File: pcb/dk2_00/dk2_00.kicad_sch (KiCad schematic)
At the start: 6 parts, among them J1 Micro_SD_Card, J7 Conn_01x01_Pin, J8 Conn_01x01_Pin, J9 Conn_01x01_Pin, SW1 SW_Push, U1 Pico

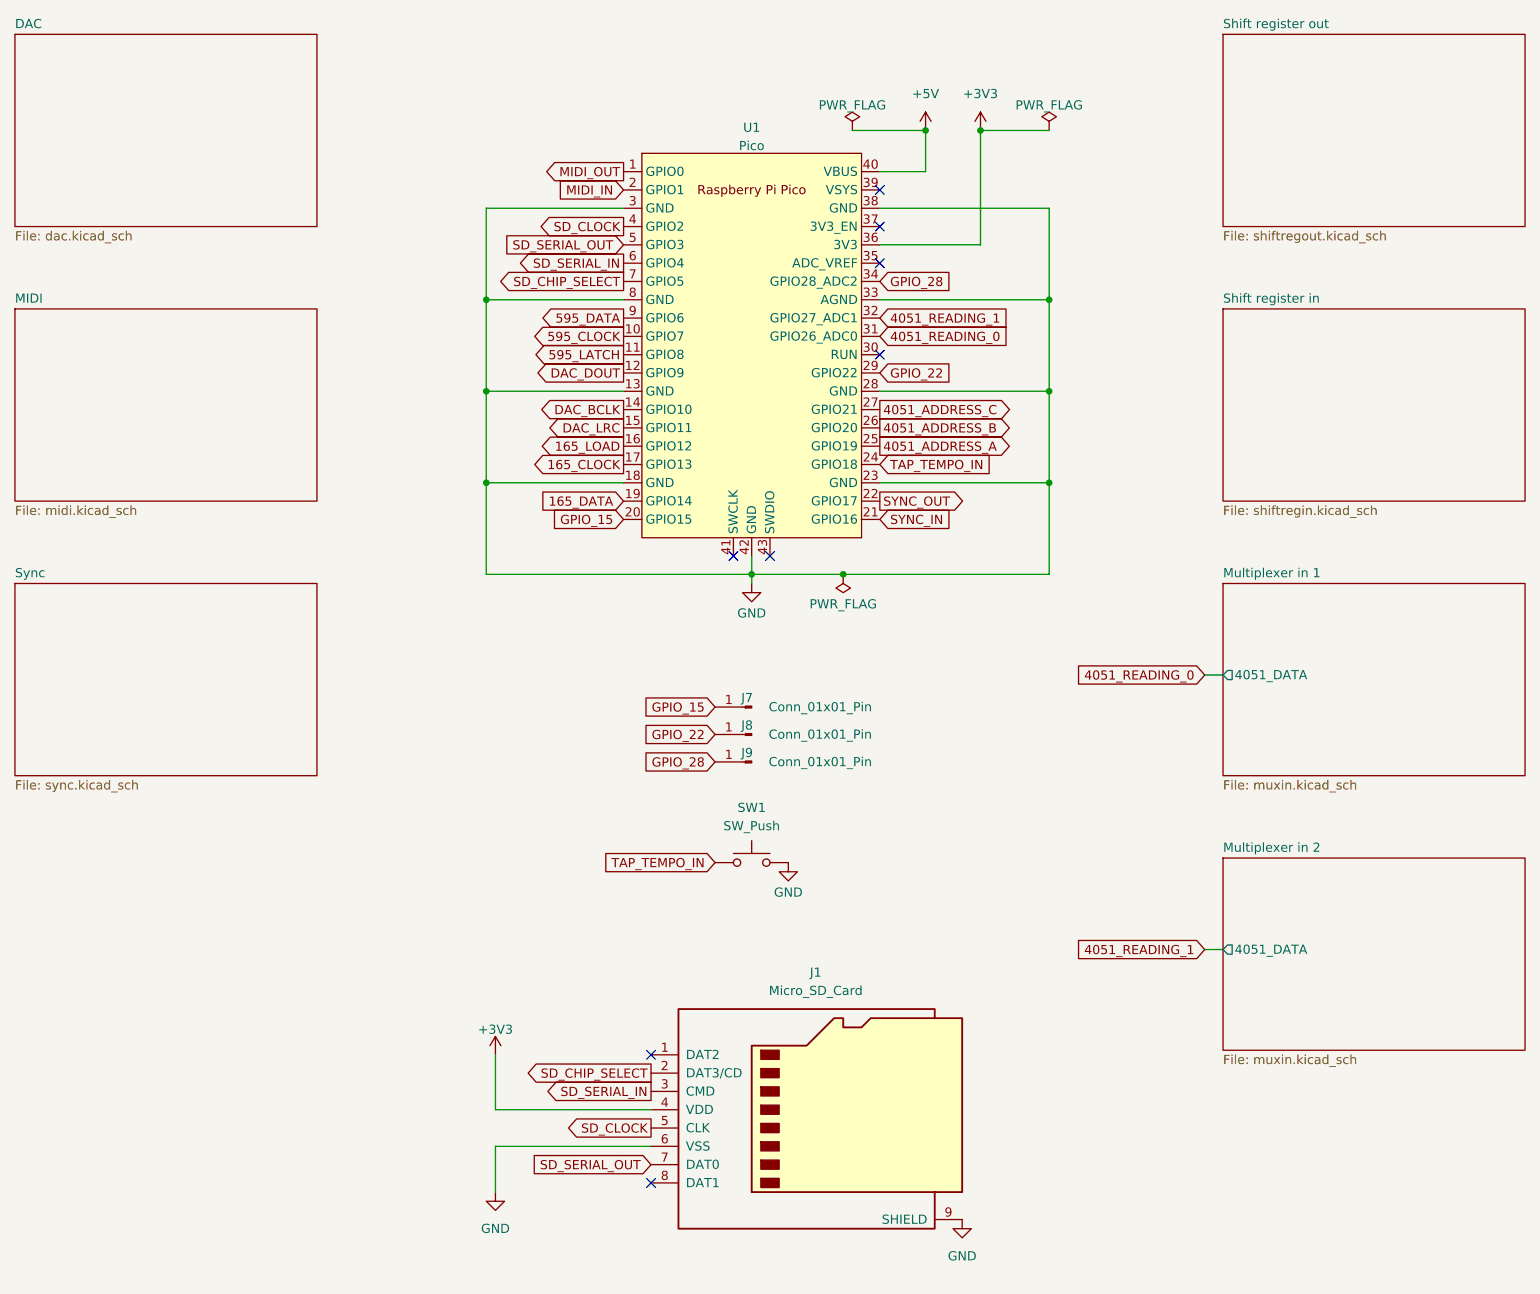
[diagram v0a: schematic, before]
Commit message: not many errors
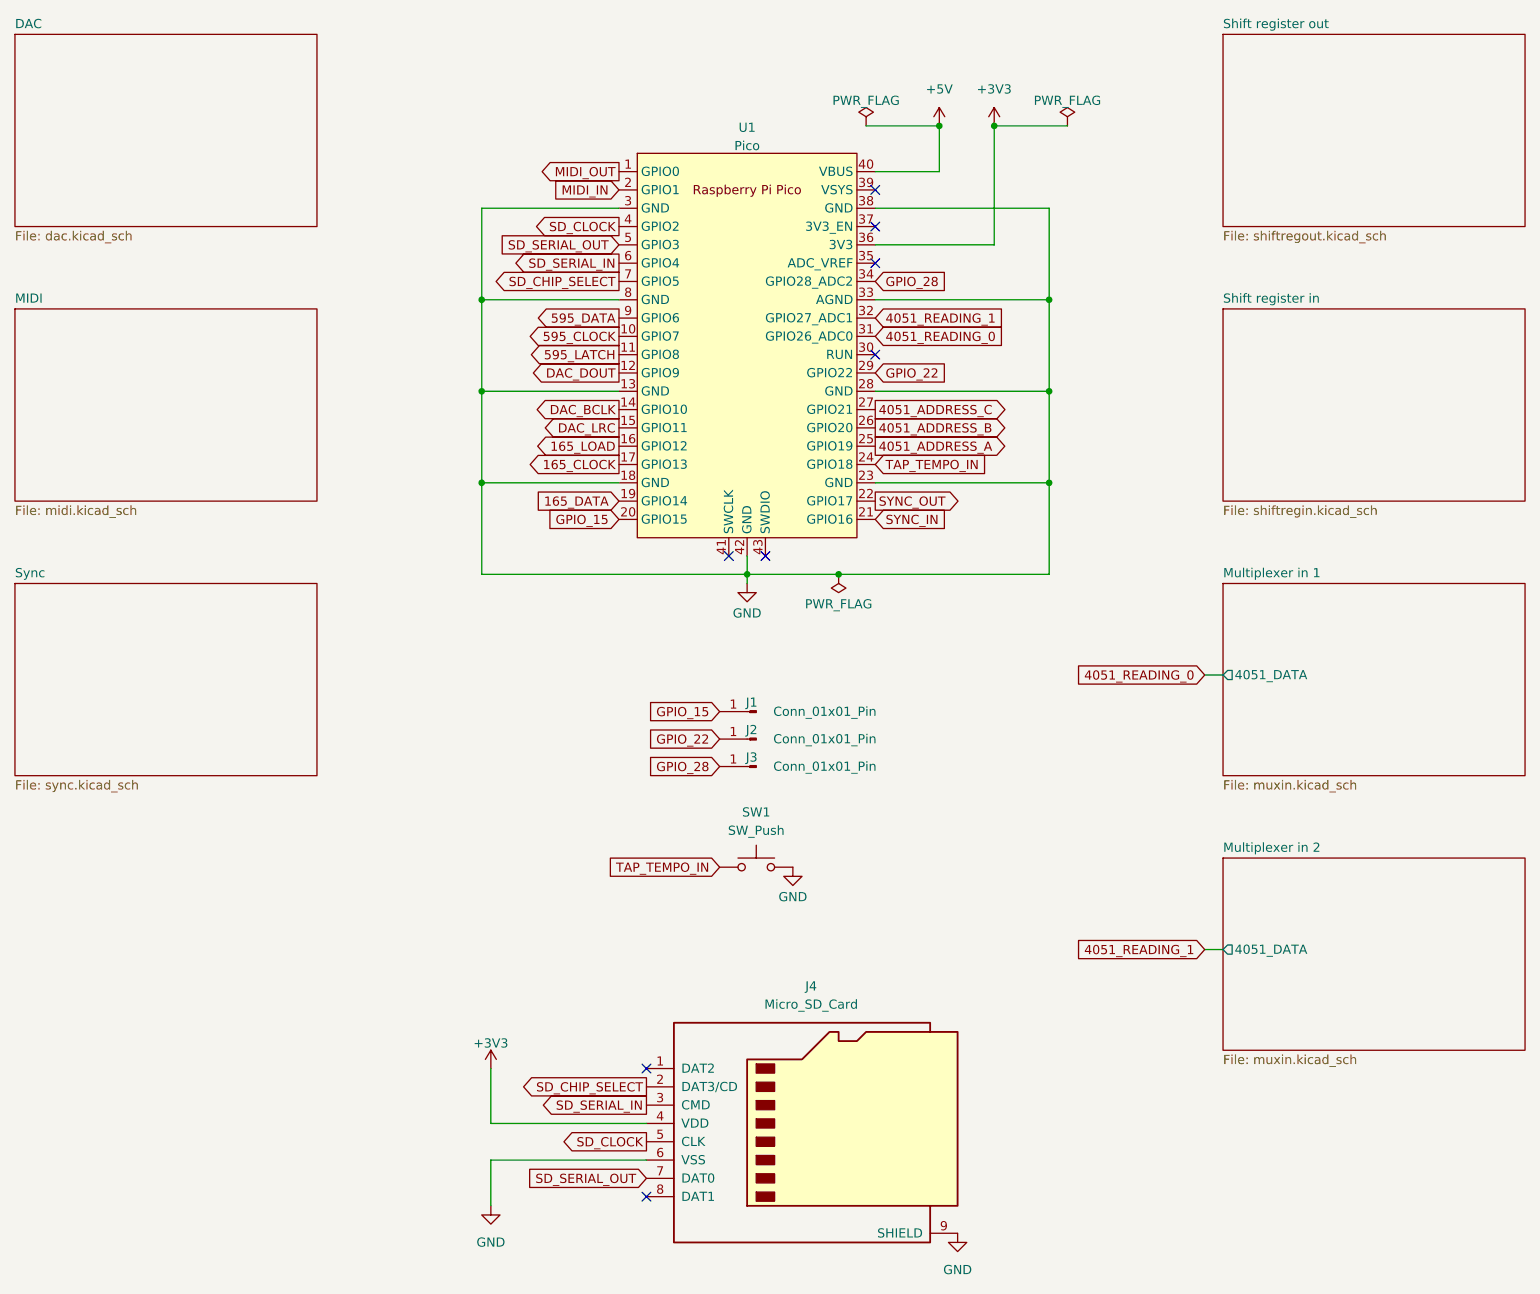
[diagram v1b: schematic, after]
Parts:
- renumbered J7 to J1, J8 to J2, J9 to J3, J1 to J4
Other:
- moved on the sheet: J1, J2, J3, J4, SW1, U1

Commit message: footprints assigned
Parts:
- J1, J2, J3: footprint (none) -> Connector_PinHeader_2.54mm:PinHeader_1x01_P2.54mm_Vertical
- J4: footprint (none) -> Connector_Card:microSD_HC_Molex_47219-2001
- SW1: footprint (none) -> Button_Switch_THT:SW_PUSH_6mm
- U1: footprint RPi_Pico:RPi_Pico_SMD_TH -> MCU_RaspberryPi_and_Boards:RPi_Pico_SMD_TH
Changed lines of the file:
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@@
       (effects (font (size 1.27 1.27)))
     )
-    (property "Footprint" "RPi_Pico:RPi_Pico_SMD_TH" (at 151.13 67.31 90)
+    (property "Footprint" "MCU_RaspberryPi_and_Boards:RPi_Pico_SMD_TH" (at 151.13 67.31 90)
       (effects (font (size 1.27 1.27)) hide)
     )
@@
       (effects (font (size 1.27 1.27)))
     )
-    (property "Footprint" "" (at 152.4 118.11 0)
+    (property "Footprint" "Connector_PinHeader_2.54mm:PinHeader_1x01_P2.54mm_Vertical" (at 152.4 118.11 0)
       (effects (font (size 1.27 1.27)) hide)
     )
@@
       (effects (font (size 1.27 1.27)))
     )
-    (property "Footprint" "" (at 152.4 125.73 0)
+    (property "Footprint" "Connector_PinHeader_2.54mm:PinHeader_1x01_P2.54mm_Vertical" (at 152.4 125.73 0)
       (effects (font (size 1.27 1.27)) hide)
     )
@@
       (effects (font (size 1.27 1.27)))
     )
-    (property "Footprint" "" (at 152.4 121.92 0)
+    (property "Footprint" "Connector_PinHeader_2.54mm:PinHeader_1x01_P2.54mm_Vertical" (at 152.4 121.92 0)
       (effects (font (size 1.27 1.27)) hide)
     )
@@
       (effects (font (size 1.27 1.27)))
     )
-    (property "Footprint" "" (at 152.4 134.62 0)
+    (property "Footprint" "Button_Switch_THT:SW_PUSH_6mm" (at 152.4 134.62 0)
       (effects (font (size 1.27 1.27)) hide)
     )
@@
       (effects (font (size 1.27 1.27)))
     )
-    (property "Footprint" "" (at 189.23 167.64 0)
-      (effects (font (size 1.27 1.27)) hide)
-    )
+    (property "Footprint" "Connector_Card:microSD_HC_Molex_47219-2001" (at 189.23 167.64 0)
+      (effects (font (size 1.27 1.27)) hide)
+    )
